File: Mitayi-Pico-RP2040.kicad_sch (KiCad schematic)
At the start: 52 parts, among them J1 USB_C_Receptacle_USB2.0, J2 Header_1, J3 Header_2, J4 USB Boot, J5 SWD, J6 USB_B_Micro, SW1 Reset, U1 NCP1117-3.3_SOT223, U2 MIC5219-3.3YM5, U3 W25Q128JVS, U4 RP2040, Y1 ABLS-12.000MHZ-B4-T

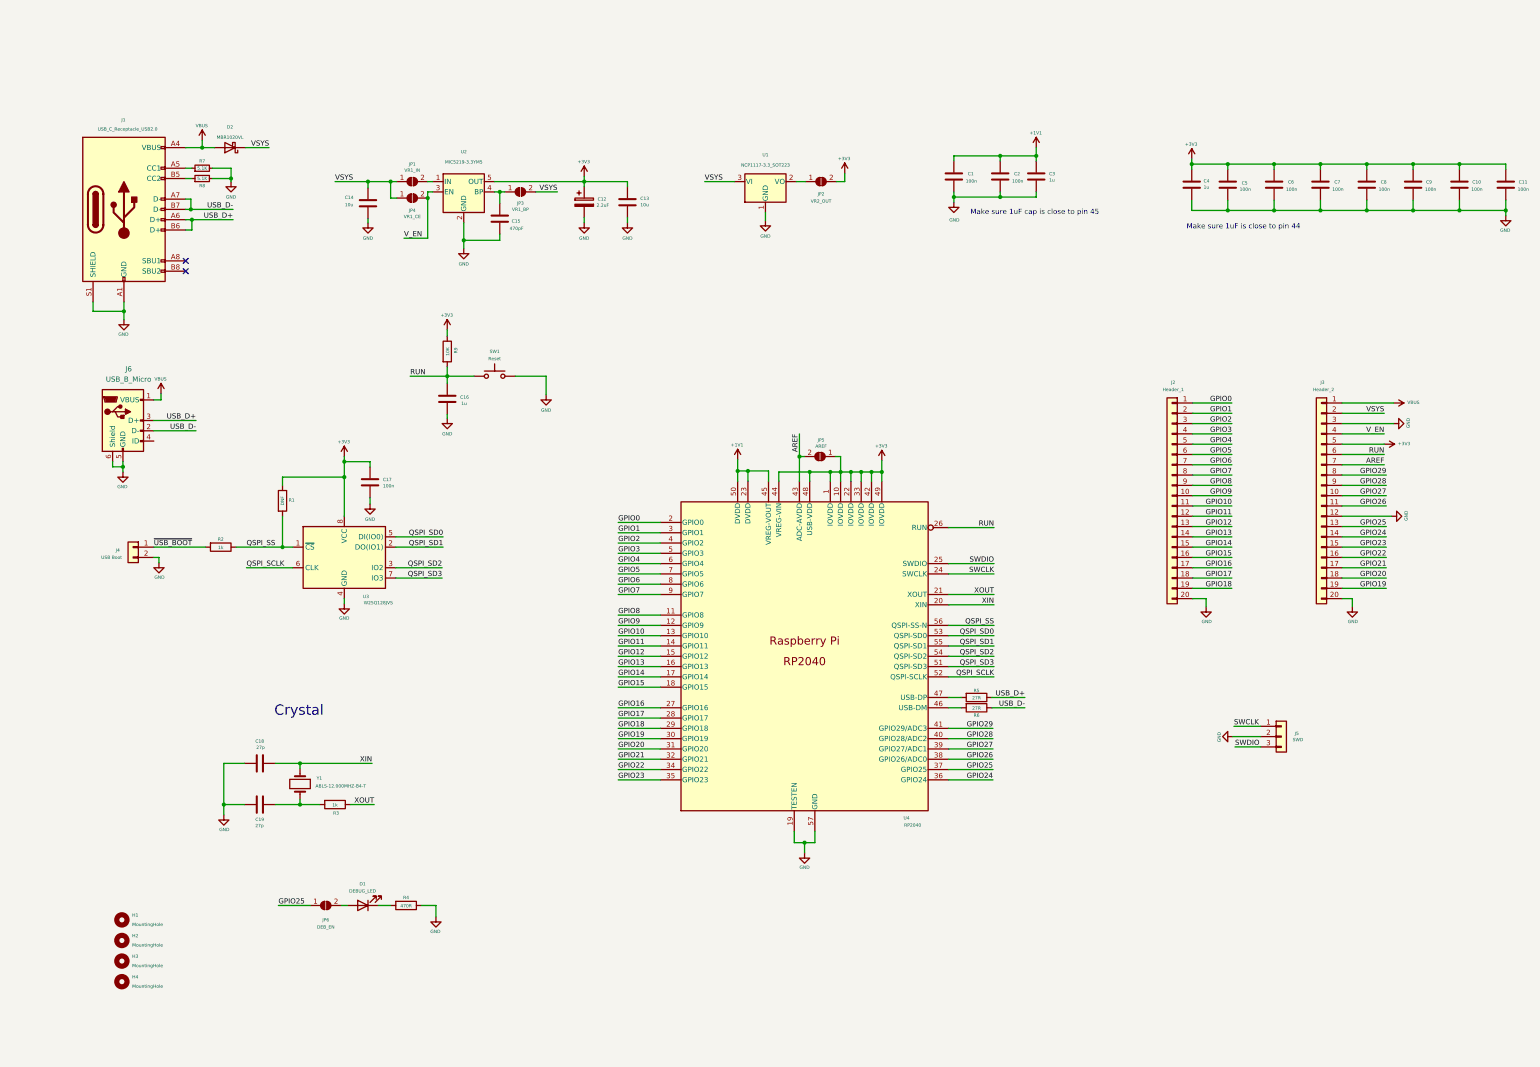
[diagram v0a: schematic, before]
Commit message: Updated root design files
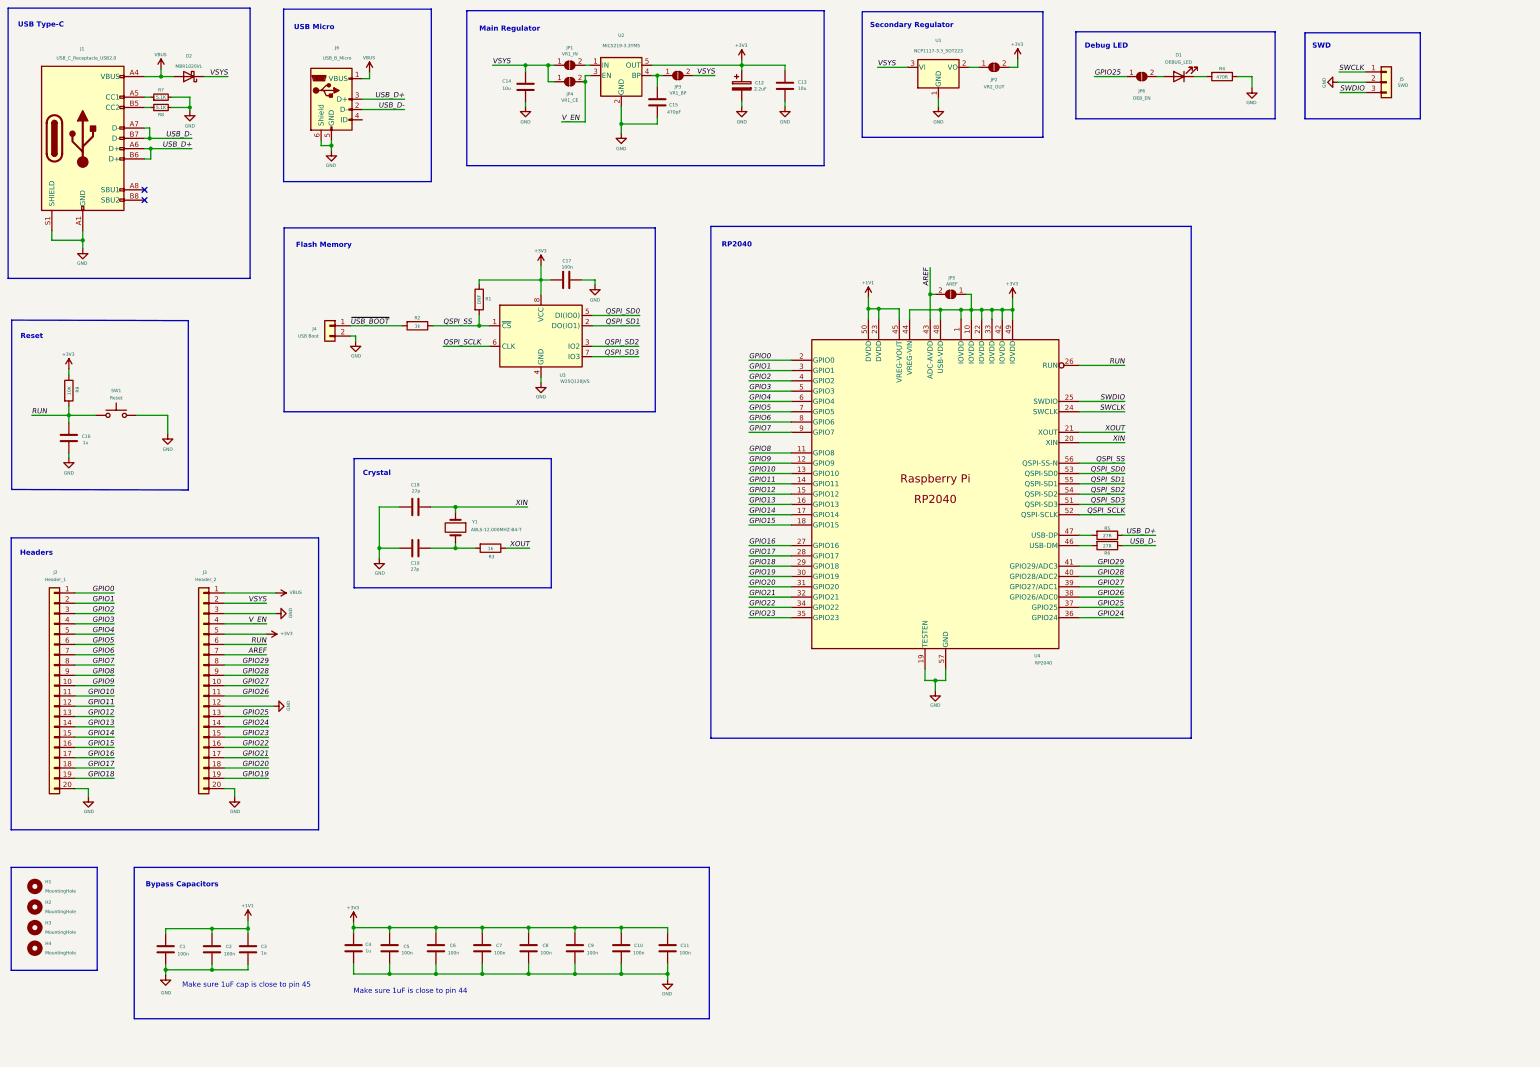
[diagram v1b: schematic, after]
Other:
- note added: "Bypass Capacitors"
- note added: "Debug LED"
- note added: "Flash Memory"
- note added: "Headers"
- note added: "Main Regulator"
- note added: "RP2040"
- note added: "Reset"
- note added: "SWD"
- note added: "Secondary Regulator"
- note added: "USB Micro"
- note added: "USB Type-C"
- moved on the sheet: C1, C10, C11, C12, C13, C14, C15, C16, C17, C18, C19, C2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

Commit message: Updated design info
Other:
- company: CIRCUITSTATE Electronics -> CIRCUITSTATE Electronics LLP
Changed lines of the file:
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@@
   (title_block
     (title "Mitayi Pico - RP2040")
-    (date "2021-08-26")
+    (date "2022-08-19")
     (rev "0.2")
-    (company "CIRCUITSTATE Electronics")
+    (company "CIRCUITSTATE Electronics LLP")
     (comment 1 "Designed by Vishnu Mohanan")
-    (comment 2 "Copyright 2021 CIRCUITSTATE Electronics")
+    (comment 2 "Copyright 2021 CIRCUITSTATE Electronics LLP")
   )
   (junction (at 136.652 245.745) (diameter 1.016) (color 0 0 0 0)

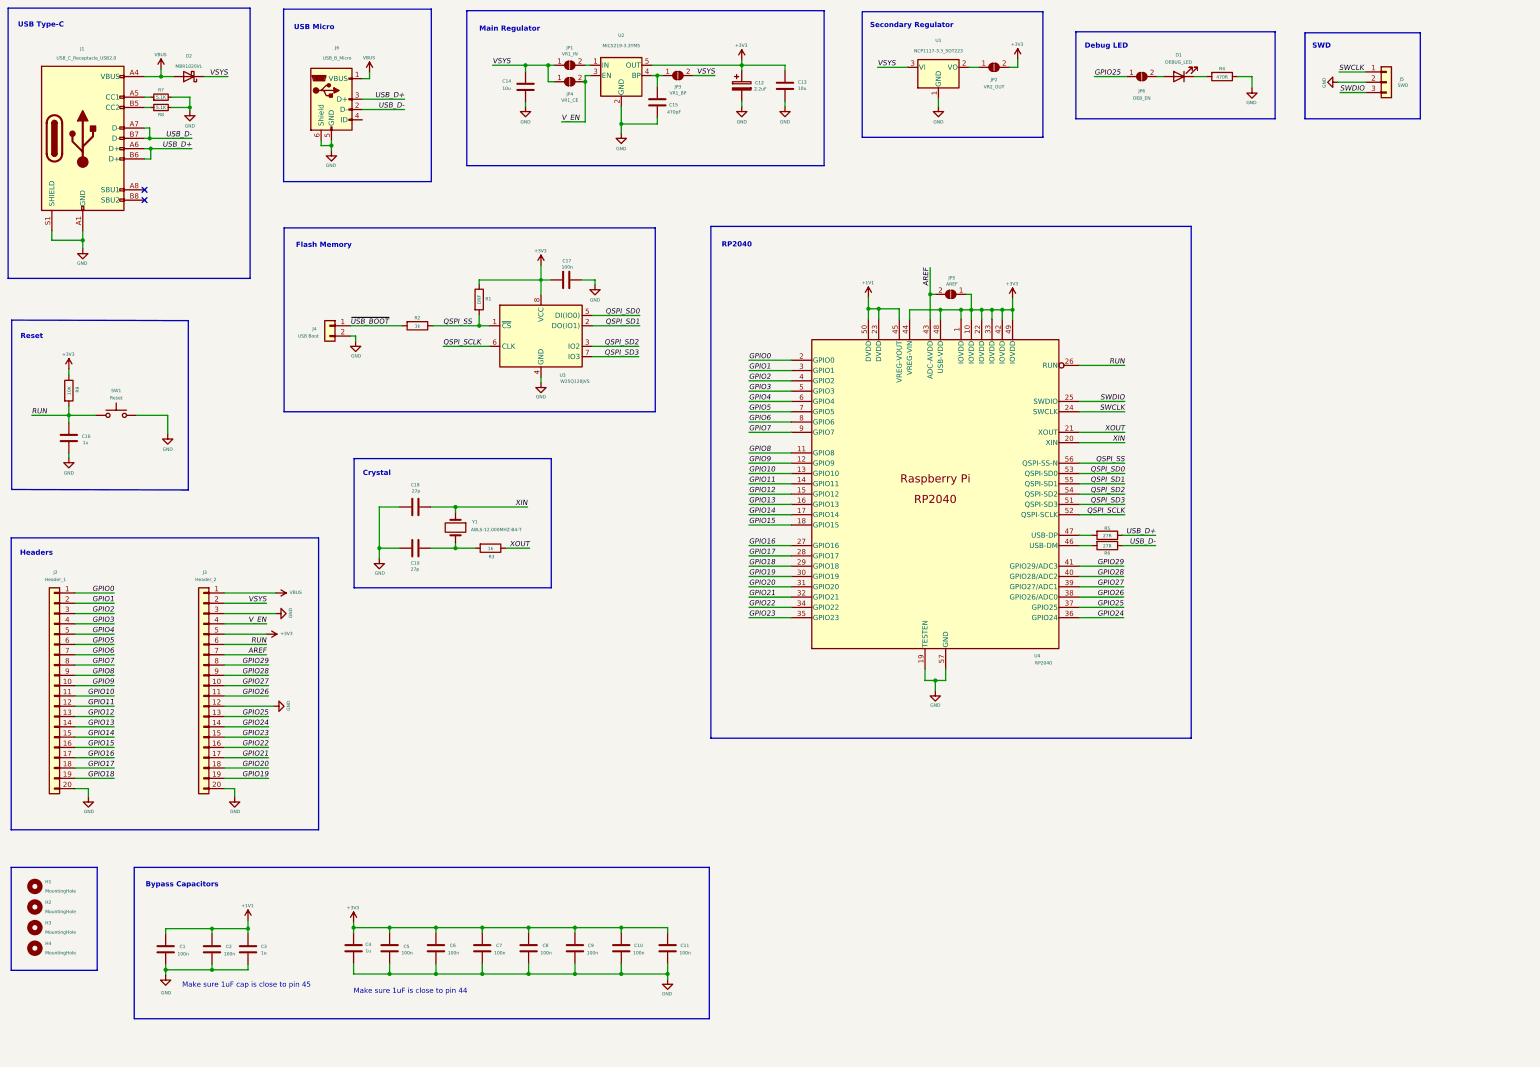
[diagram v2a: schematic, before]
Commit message: r0.3
Connected with CADLAB.io
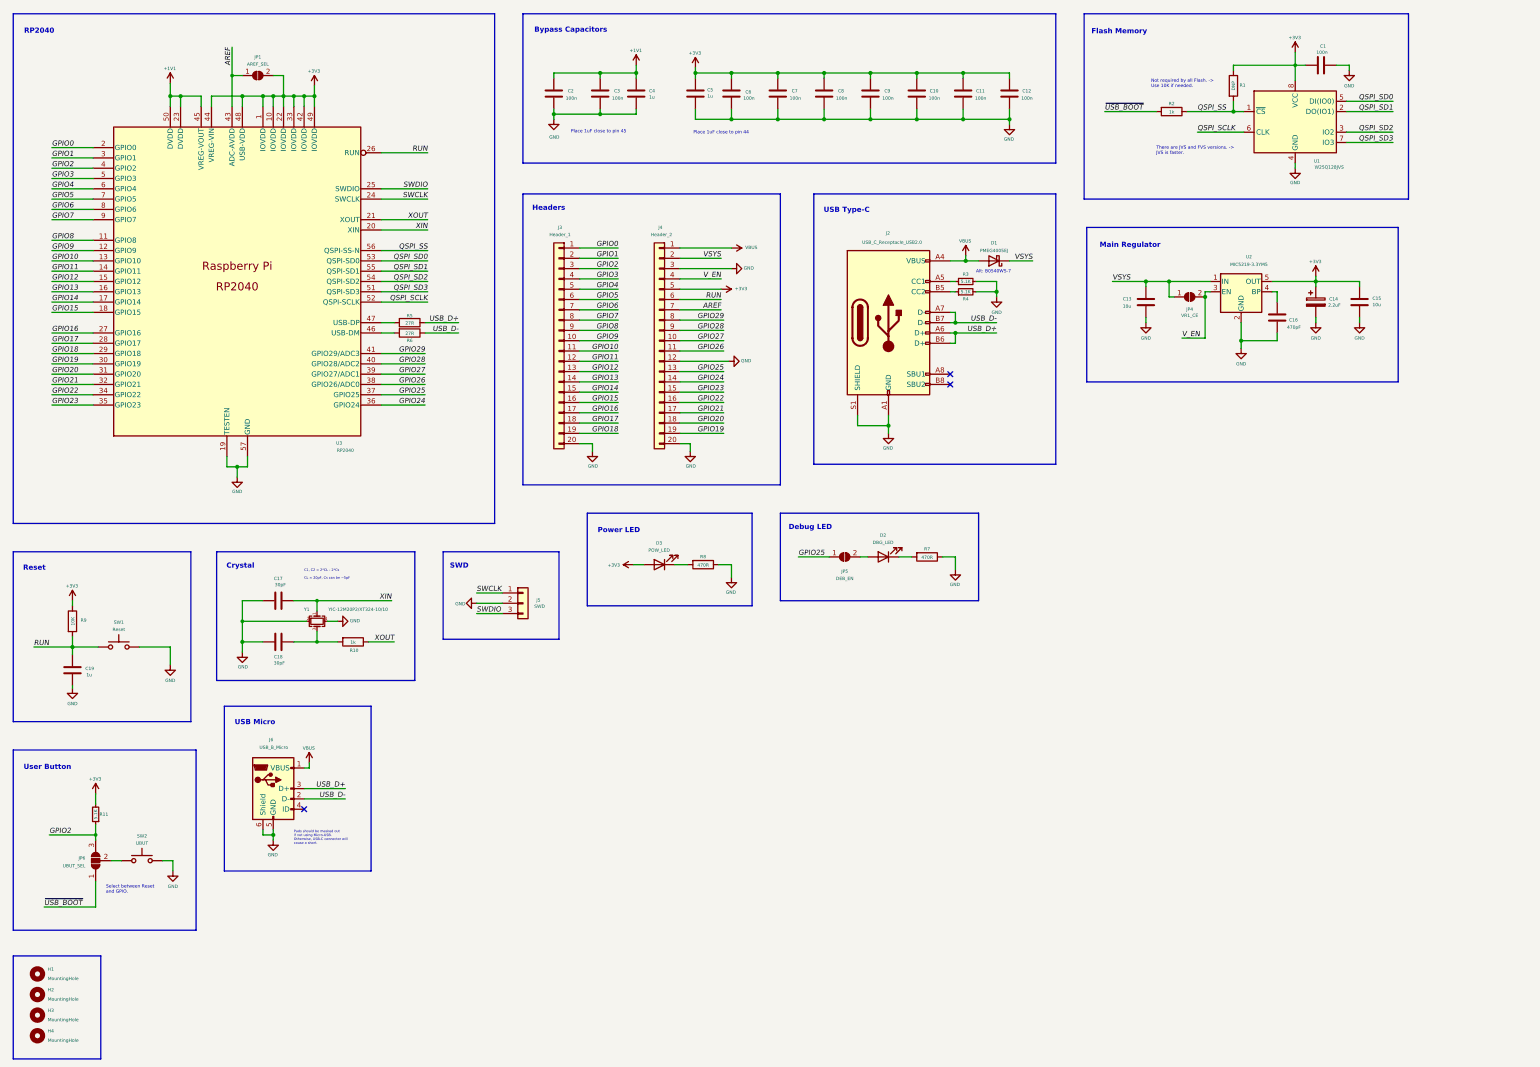
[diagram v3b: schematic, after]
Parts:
- removed J4: USB Boot, Resistor_SMD:R_0603_1608Metric_Pad0.98x0.95mm_HandSolder, symbol Connector_Generic:Conn_01x02
- removed JP2: VR2_OUT, Resistor_SMD:R_0402_1005Metric, symbol Jumper:SolderJumper_2_Open
- removed JP3: VR1_BP, Resistor_SMD:R_0402_1005Metric, symbol Jumper:SolderJumper_2_Open
- removed JP5: AREF, Resistor_SMD:R_0402_1005Metric, symbol Jumper:SolderJumper_2_Open
- removed U1: NCP1117-3.3_SOT223, Package_TO_SOT_SMD:SOT-223-3_TabPin2, symbol Regulator_Linear:NCP1117-3.3_SOT223
- removed Y1: ABLS-12.000MHZ-B4-T, Crystal:Crystal_SMD_3225-4Pin_3.2x2.5mm, symbol Device:Crystal
- added D3: POW_LED, LED_SMD:LED_0603_1608Metric, symbol Device:LED
- added JP6: UBUT_SEL, CIRCUITSTATE_Jumper_SMD:Solder-Jumper_3P_Open_0402, symbol Jumper:SolderJumper_3_Open
- added R11: 5.1K, Resistor_SMD:R_0402_1005Metric_Pad0.72x0.64mm_HandSolder, symbol Device:R_Small
- added R8: 470R, Resistor_SMD:R_0402_1005Metric_Pad0.72x0.64mm_HandSolder, symbol Device:R
- added SW2: UBUT, CIRCUITSTATE_Switch_SMD:CK_SW_SPST_UK-B0273-SP25Y, symbol Switch:SW_Push
- added Y1: YIC-12M20P2/XT324-10/10, Crystal:Crystal_SMD_3225-4Pin_3.2x2.5mm, symbol Device:Crystal_GND24_Small
- C17: renamed from C18; value 27p -> 30pF
- C18: renamed from C19; value 27p -> 30pF
- D1: renamed from D2; value MBR1020VL -> PMEG4005EJ; footprint Diode_SMD:D_SOD-123F -> Diode_SMD:D_SOD-323_HandSoldering
- D2: renamed from D1; value DEBUG_LED -> DBG_LED; footprint Capacitor_SMD:C_0603_1608Metric_Pad1.08x0.95mm_HandSolder -> LED_SMD:LED_0603_1608Metric
- JP1: value VR1_IN -> AREF_SEL; footprint Resistor_SMD:R_0402_1005Metric -> CIRCUITSTATE_Jumper_SMD:Solder-Jumper_2P_Open_0402
- JP4: footprint Resistor_SMD:R_0402_1005Metric -> CIRCUITSTATE_Jumper_SMD:Solder-Jumper_2P_Open_0402
- JP5: renamed from JP6; footprint Resistor_SMD:R_0402_1005Metric -> CIRCUITSTATE_Jumper_SMD:Solder-Jumper_2P_Open_0402
- R1: value DNF -> DNP
- renumbered C17 to C1, C9 to C10, C10 to C11, C11 to C12, C14 to C13, C12 to C14, C13 to C15, C15 to C16, C16 to C19, C1 to C2, C2 to C3, C3 to C4, C4 to C5, C5 to C6, C6 to C7, C7 to C8, C8 to C9, J1 to J2, J2 to J3, J3 to J4, R3 to R10, R7 to R3, R8 to R4, R4 to R7, U3 to U1, U4 to U3
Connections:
- net +3V3: now also JP1.2 (B), D3.2 (A), R11.2
- net AREF: now also JP1.1 (A)
- net GND: now also R8.1, SW2.2, Y1.2, Y1.4
- net GPIO2: now also JP6.3 (B), R11.1
- net VSYS: now also U2.1 (IN); no longer JP1.1 (A)
- net XIN: now also Y1.1
- net ~{USB_BOOT}: now also JP6.1 (A)
- net at C18.1, R10.2: now also Y1.3
- new net: D3.1 (K), R8.2
- new net: JP6.2 (C), SW2.1
- no-connect marks 2 -> 3
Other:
- note added: "Alt: B0540WS-7"
- note added: "C1, C2 = 2*CL - 2*Cs CL = 20pF, Cs can be ~5pF"
- note added: "Not required by all Flash. -> Use 10K if needed."
- note added: "Pads should be masked out if not using Micro-USB. Otherwise, USB-C connector will cause a short."
- note added: "Place 1uF close to pin 44"
- note added: "Place 1uF close to pin 45"
- note added: "Power LED"
- note added: "Select between Reset and GPIO."
- note added: "There are JVS and FVS versions. -> JVS is faster."
- note added: "User Button"
- note removed: "Make sure 1uF cap is close to pin 45"
- note removed: "Make sure 1uF is close to pin 44"
- note removed: "Secondary Regulator"
- title: Mitayi Pico - RP2040 -> Mitayi Pico - Schematic
- moved on the sheet: C1, C10, C11, C12, C13, C14, C15, C16, C17, C18, C19, C2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
